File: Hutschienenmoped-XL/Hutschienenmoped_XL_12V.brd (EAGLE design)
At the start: 96.3 x 101.8 mm, 118 parts, among them J1 638207222005, J13 638207222005, J15 638207222008, J2 645004114822, J3 61302211821, J4 61300421121, J6 61302211821, J7 638207222005, J8 638207222007, U1 ESP32-S3-DEVKITC-1-N8R2, U4 TLE9250VSJ

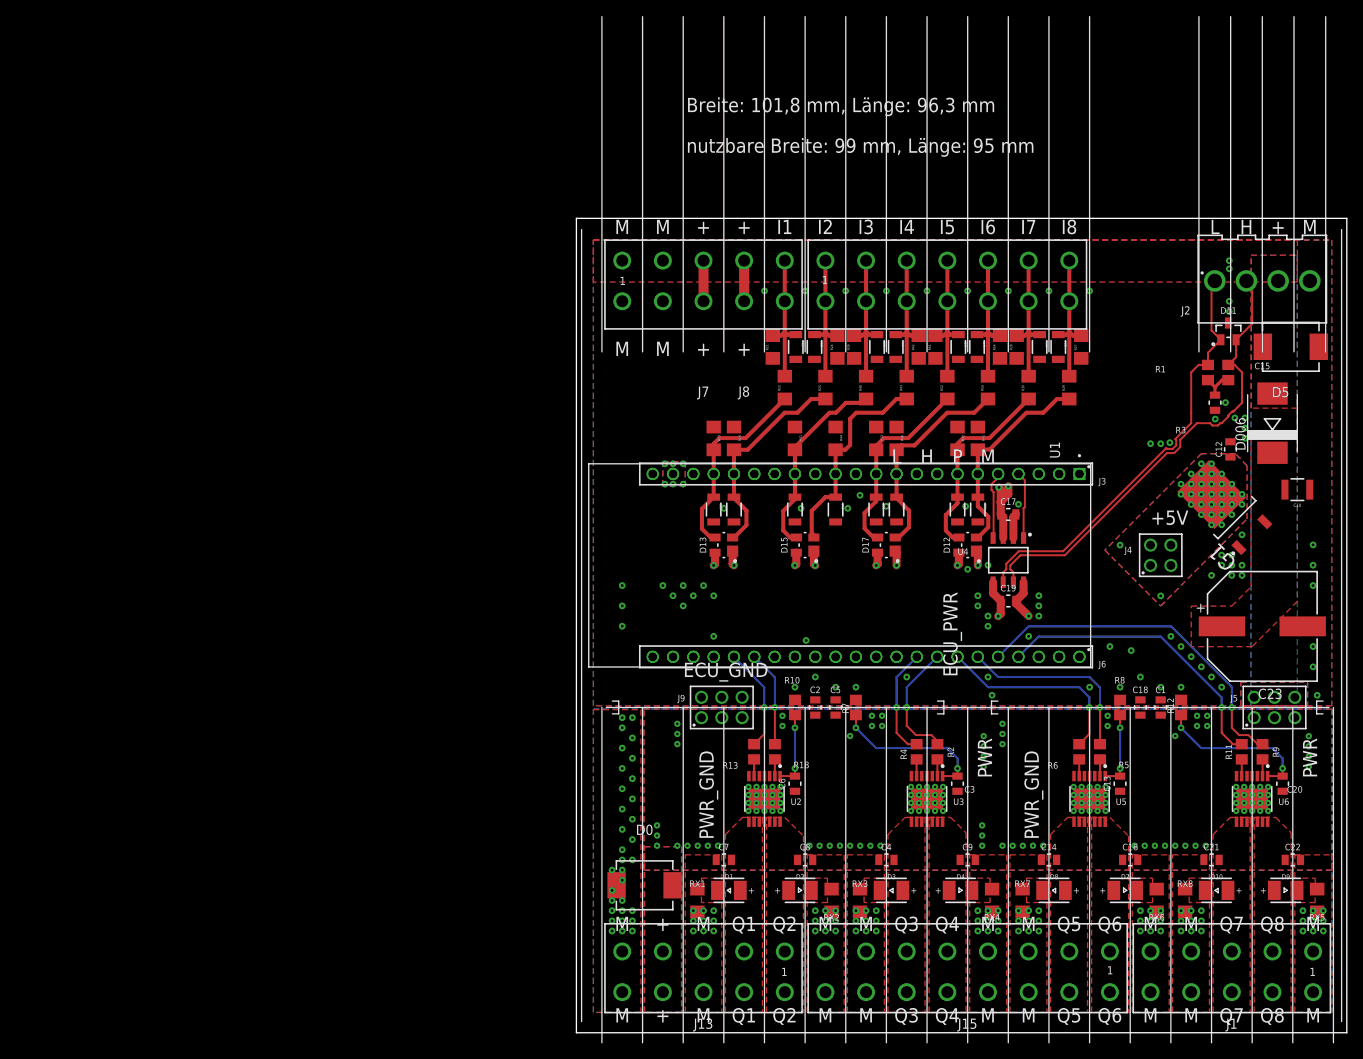
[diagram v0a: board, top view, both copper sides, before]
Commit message: NOT correct !
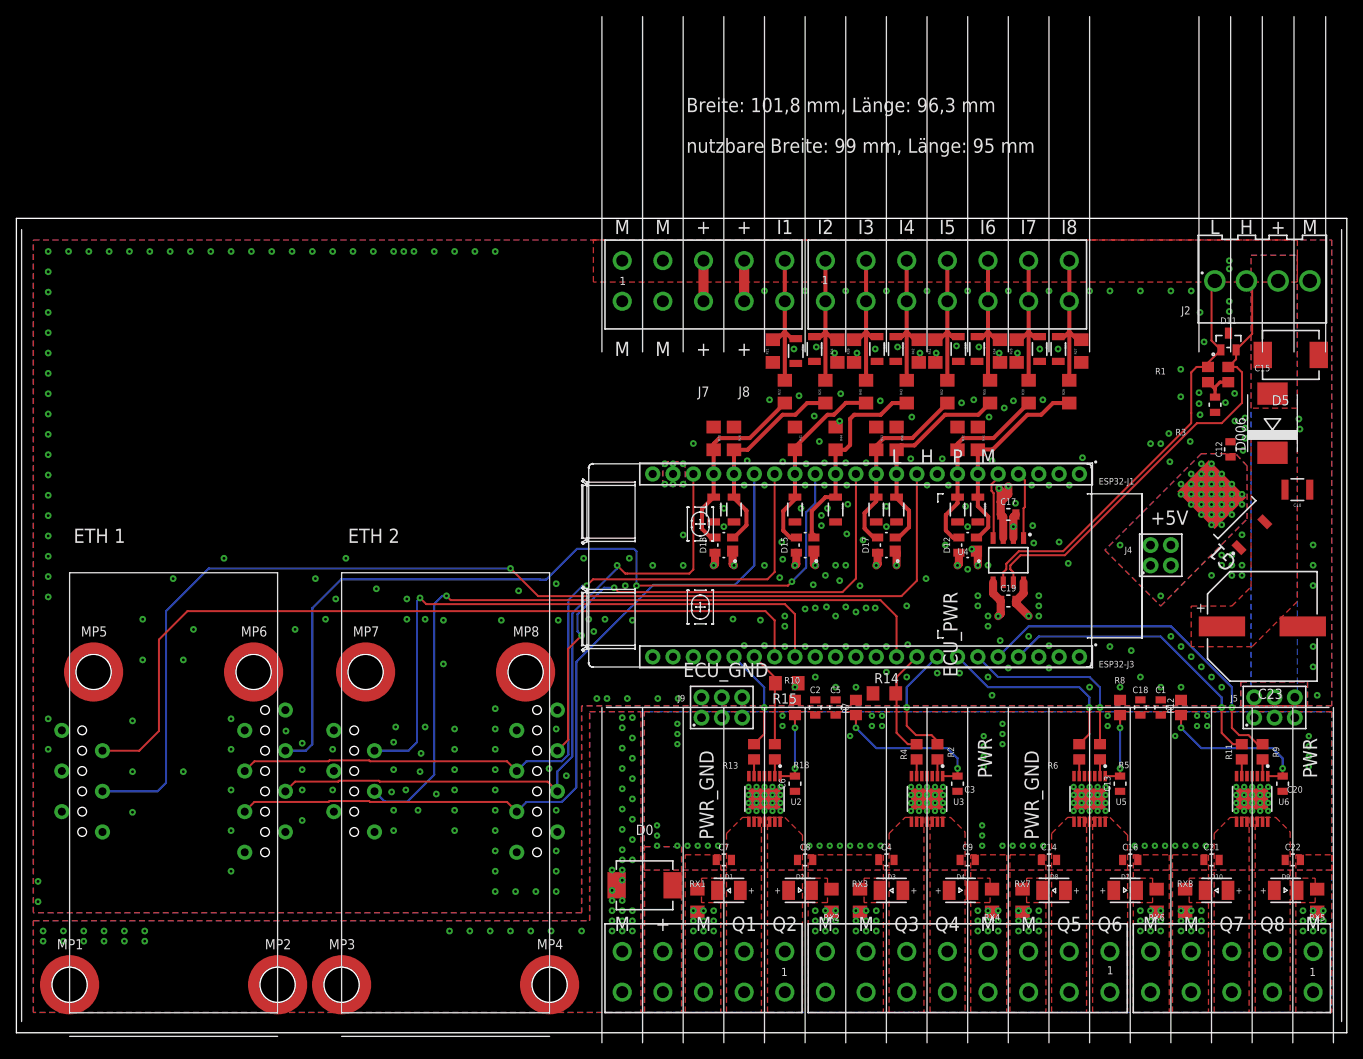
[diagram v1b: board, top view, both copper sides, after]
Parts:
- removed U1: ESP32-S3-DEVKITC-1-N8R2, ESP32-S3-DEVKITC-1-N8R2:XCVR_ESP32-S3-DEVKITC-1-N8R2
- added MP1, MP2, MP3, MP4, MP5, MP6, MP7, MP8: M3 x 2.5mm, Wurth_Assembly_WA-SMSI:WA-SMSI_9774025360
- added R14, R15: 13K, resistor:R1206
- added W1-J1, W2-J1: 61301015721, WE-special:61301015721
- added W1-J2, W2-J2: 61300615721, Wurth_Connectors_WR-PHD:61300615721
- moved D11 1.27 mm to (80.9, 86.4)
- moved D5 1.02 mm to (88.6, 84.7)
- moved R55 0.57 mm to (51.1, 80.1)
- moved C31 0.51 mm to (26.8, 85.2)
- moved R21 0.51 mm to (23.9, 85.2)
- moved R22 0.51 mm to (25.4, 80.1)
- moved R24 0.51 mm to (32.0, 85.2)
- moved R25 0.51 mm to (30.5, 80.1)
- moved R27 0.51 mm to (62.5, 85.2)
- moved R28 0.51 mm to (54.4, 85.2)
- moved R29 0.51 mm to (61.0, 80.1)
- moved R30 0.51 mm to (55.9, 80.1)
- moved R39 0.51 mm to (34.1, 85.2)
- moved R40 0.51 mm to (35.6, 80.1)
- moved R42 0.51 mm to (42.1, 85.2)
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- renumbered J3 to ESP32-J1, J6 to ESP32-J3
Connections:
- removed net IX00: U1.J1_20
- removed net IX06: U1.J1_8
- removed net MB_UART_RTS1: U1.J1_16
- removed net MB_UART_RXD1: U1.J1_12
- removed net MB_UART_RXD2: U1.J1_17
- removed net N$20: J13.5, J13.A5
- removed net QX06: U1.J3_16
- removed net QX07: U1.J3_10
- new net CS0: ESP32-J1.14, W1-J1.6
- new net CS1: ESP32-J1.12, W2-J1.6
- new net INT0: ESP32-J3.16, W1-J2.5
- new net INT1: ESP32-J3.15, W2-J2.5
- new net MISO: ESP32-J1.20, W1-J1.4, W2-J1.4
- new net MOSI: ESP32-J1.17, W1-J1.3, W2-J1.3
- new net RST0: ESP32-J1.9, W1-J2.3
- new net RST1: ESP32-J3.10, W2-J2.3
- new net SCLK: ESP32-J1.16, W1-J1.5, W2-J1.5
- net +3V3: now also ESP32-J1.1, ESP32-J1.2, W1-J1.7, W1-J1.8, W1-J2.1, W2-J1.7, W2-J1.8, W2-J2.1; no longer U1.J1_1, U1.J1_2
- net +5V: now also ESP32-J1.21; no longer U1.J1_21
- net BOOT: now also ESP32-J3.14; no longer U1.J3_14
- net CAN1_RXD: now also ESP32-J1.5; no longer U1.J1_5
- net CAN1_TXD: now also ESP32-J1.4; no longer U1.J1_4
- net CI1: now also ESP32-J1.19; no longer U1.J1_19
- net CI2: now also ESP32-J1.18; no longer U1.J1_18
- net CI3: now also ESP32-J1.15; no longer U1.J1_15
- net CI4: now also ESP32-J1.13; no longer U1.J1_13
- net CI5: now also ESP32-J1.11; no longer U1.J1_11
- net CI6: now also ESP32-J1.10; no longer U1.J1_10
- net CI7: now also ESP32-J1.7; no longer U1.J1_7
- net CI8: now also ESP32-J1.6; no longer U1.J1_6
- net ECU_GND: now also ESP32-J1.22, ESP32-J3.1, ESP32-J3.21, ESP32-J3.22, MP5.1, MP6.1, MP7.1, MP8.1, R14.1, R15.1, W1-J1.1, W1-J1.2, W1-J2.6, W2-J1.1, W2-J1.2, W2-J2.6; no longer U1.J1_22, U1.J3_1, U1.J3_21, U1.J3_22
- net PWR_GND: now also J13.5, J13.A5, MP1.1, MP2.1, MP3.1, MP4.1
- net Q1C: now also ESP32-J3.18; no longer U1.J3_18
- net Q2C: now also ESP32-J3.17, R15.2; no longer U1.J3_17
- net Q3C: now also ESP32-J3.9, R14.2; no longer U1.J3_9
- net Q4C: now also ESP32-J3.8; no longer U1.J3_8
- net Q5C: now also ESP32-J3.7; no longer U1.J3_7
- net Q6C: now also ESP32-J3.6; no longer U1.J3_6
- net Q7C: now also ESP32-J3.4; no longer U1.J3_4
- net Q8C: now also ESP32-J3.5; no longer U1.J3_5
- net RESET: now also ESP32-J1.3; no longer U1.J1_3
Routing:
- net RST0: track 0.00 -> 141.5 mm, vias 0 -> 1
- net CS0: track 0.00 -> 103.1 mm, vias 0 -> 2
- net INT0: track 0.00 -> 103.0 mm
- net SCLK: track 0.00 -> 101.2 mm, vias 0 -> 1
- net MOSI: track 0.00 -> 98.2 mm
- net RST1: track 0.00 -> 95.1 mm, vias 0 -> 1
- net MISO: track 0.00 -> 88.5 mm, vias 0 -> 1
- net INT1: track 0.00 -> 77.0 mm, vias 0 -> 1
- net CS1: track 0.00 -> 68.7 mm, vias 0 -> 2
- net Q3C: track 13.7 -> 15.7 mm, vias 1 -> 0
- net I6: track 17.7 -> 18.6 mm
- net I1: track 17.7 -> 18.6 mm
- net I2: track 17.7 -> 18.5 mm
- net I7: track 17.7 -> 18.5 mm
- net I4: track 17.7 -> 18.5 mm
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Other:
- board size 96.3 x 101.8 mm -> 166.3 x 101.8 mm
- board text added: "ETH 1"
- board text added: "ETH 2"
